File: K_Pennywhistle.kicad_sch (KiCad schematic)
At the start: 67 parts, among them J1 Bias Control, J2 Conn_Coaxial, J3 P IN, J4 Conn_Coaxial, Q1 RD15HVF1, Q2 RD15HVF1, Q3 ZVP2106G, T1 BN43-302, T2 TLT BN43-202, T3 Output, U1 UA78M06CKVURG3

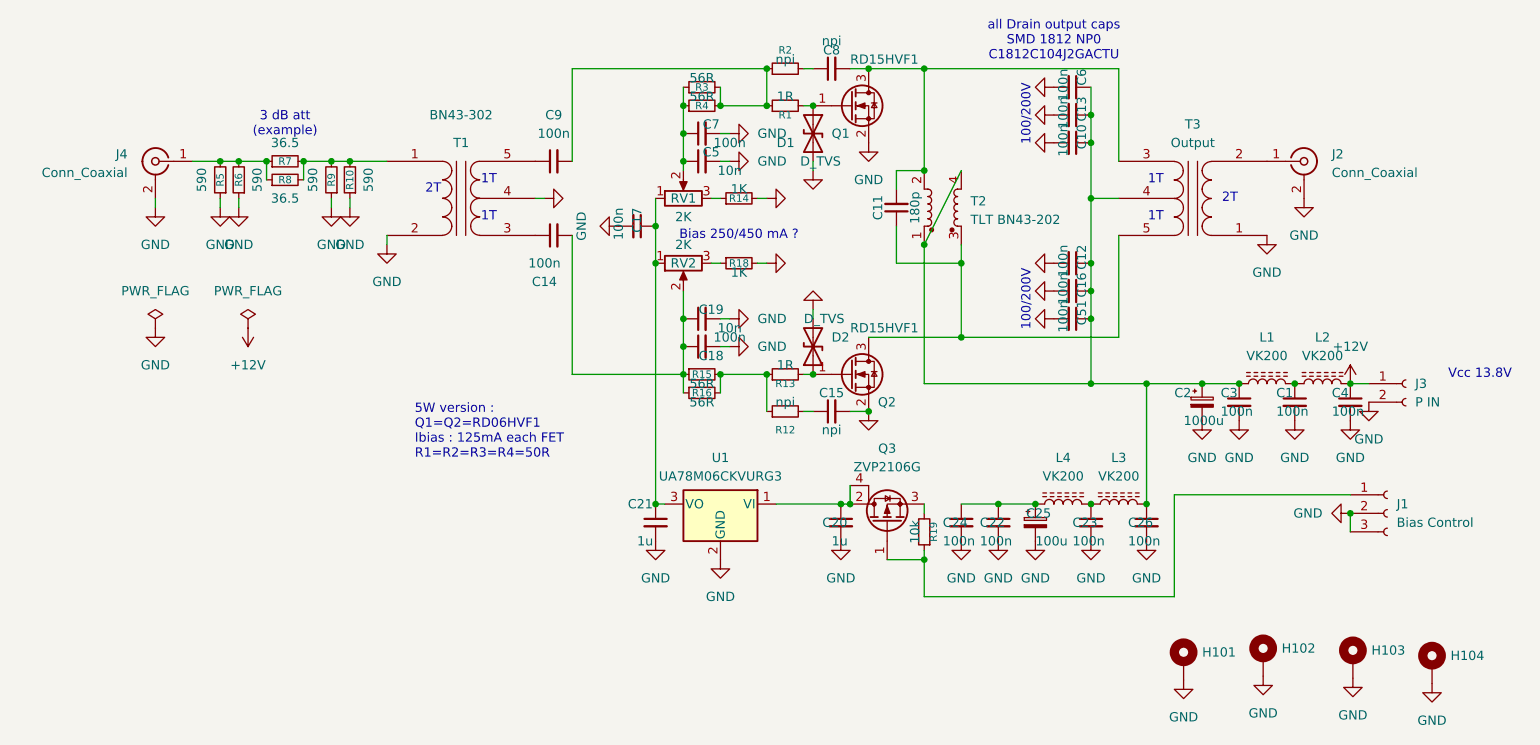
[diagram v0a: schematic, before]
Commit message: first routed draft, fix some errors
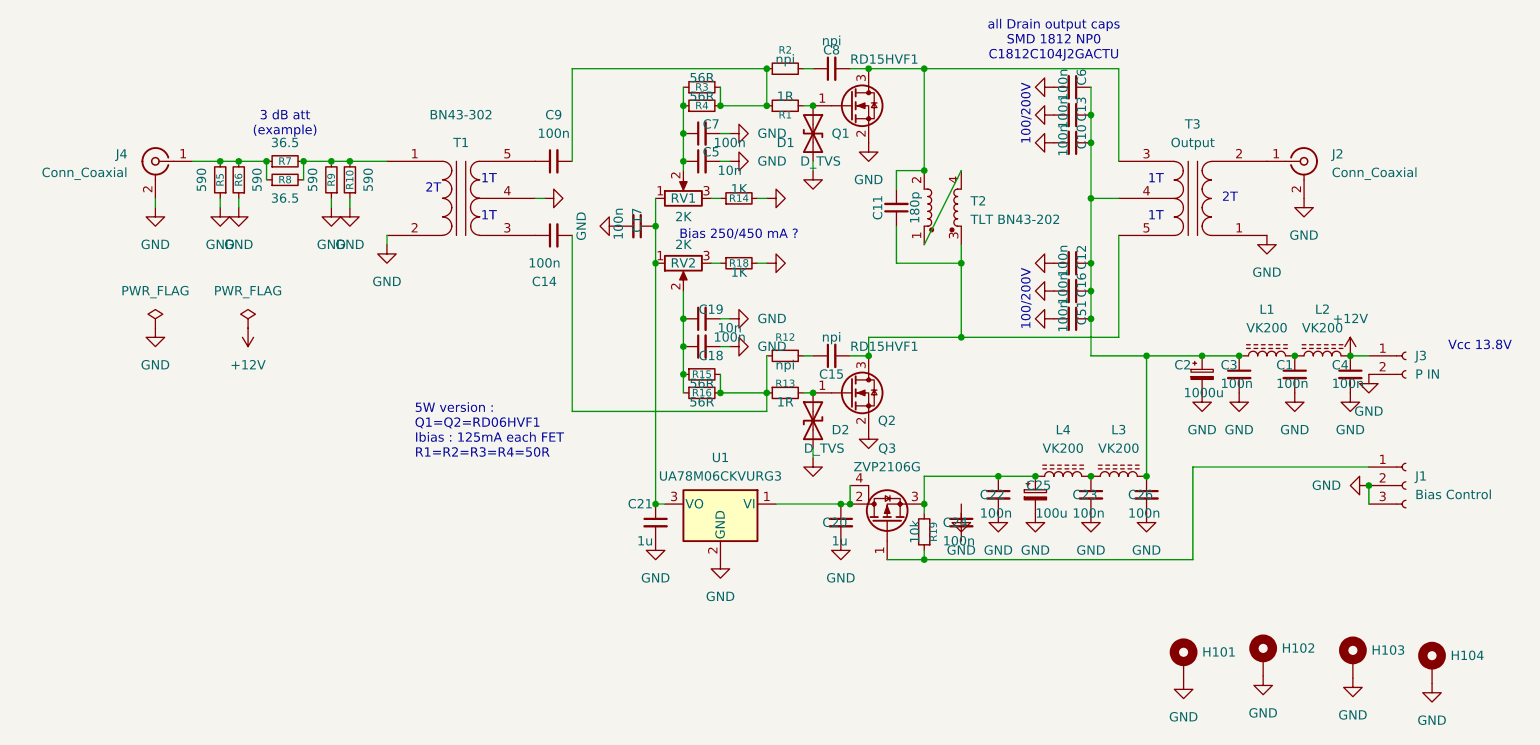
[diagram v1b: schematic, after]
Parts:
- D1, D2: footprint (none) -> Diode_SMD:D_0805_2012Metric
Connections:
- net GND: no longer C15.2, C24.2
- net at C10.1, C12.1, C13.1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: no longer T2.1, T2.4
- net at Q3.3 (S), R19.2: now also C22.1, C25.1, L4.1
- net at C11.1, Q2.3 (D), T2.3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: now also C15.2
- net at R12.1, R13.1, R15.2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: now also C14.2
- net at C18.1, C19.1, R15.1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: no longer C14.2
- new net: T2.1, T2.4
- now unconnected: C24.1
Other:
- moved on the sheet: C1, C15, C2, C22, C23, C25, C26, C3, C4, D2, J1, J3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
